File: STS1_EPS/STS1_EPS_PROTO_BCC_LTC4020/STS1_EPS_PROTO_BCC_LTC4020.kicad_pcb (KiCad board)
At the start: 2 copper layers, 47 parts, among them J1 1729267, J10 External Thermistor, J11 Terminal BAT, J9 Output, Q1 SI7135DP-T1-GE3, U1 LTC4020EUHF-PBF, U2 SI7272DP-T1-GE3, U3 SI7272DP-T1-GE3

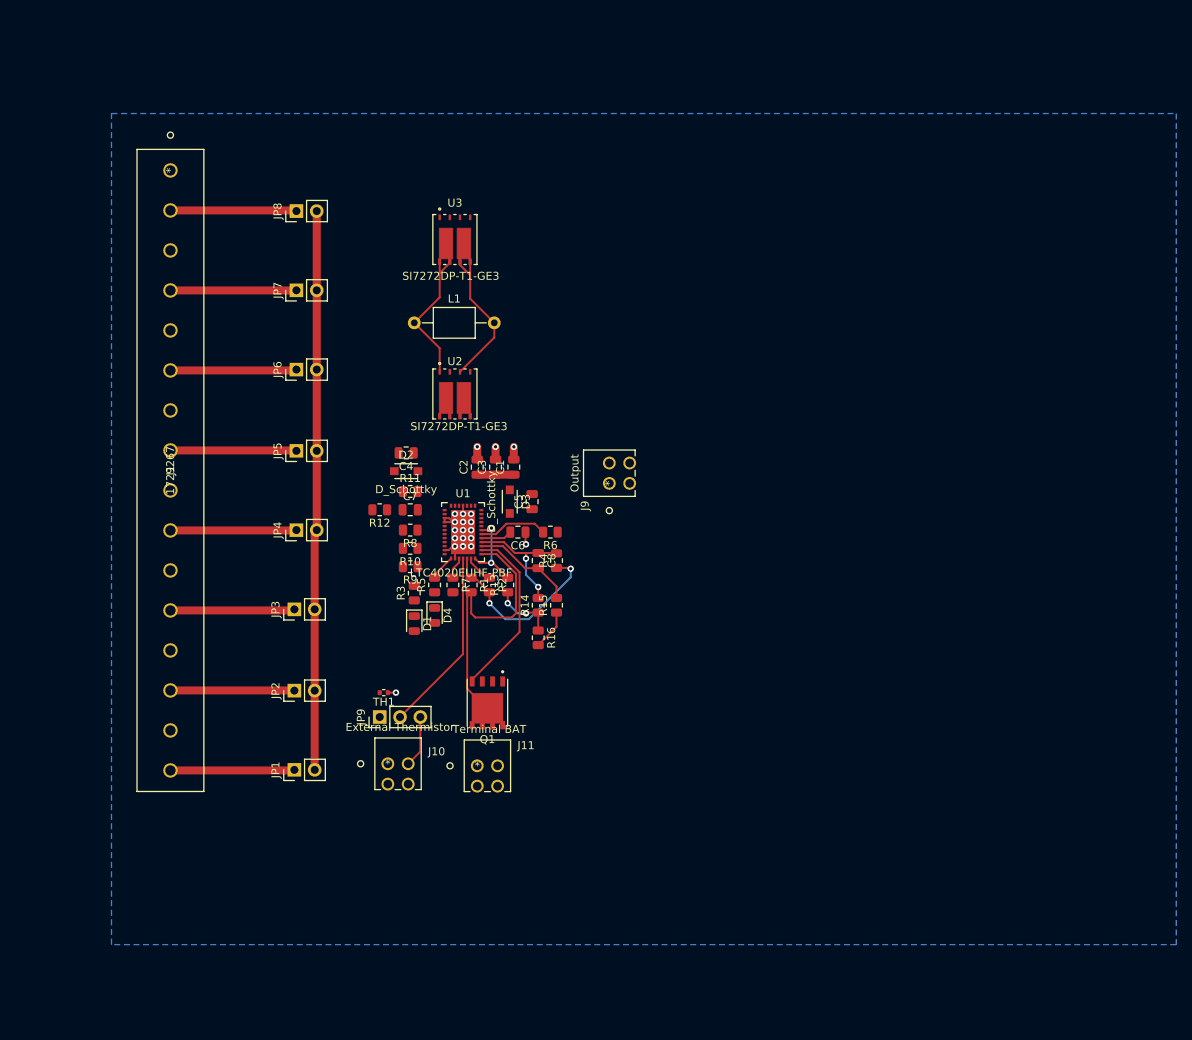
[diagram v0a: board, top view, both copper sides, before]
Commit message: Reworked BCC
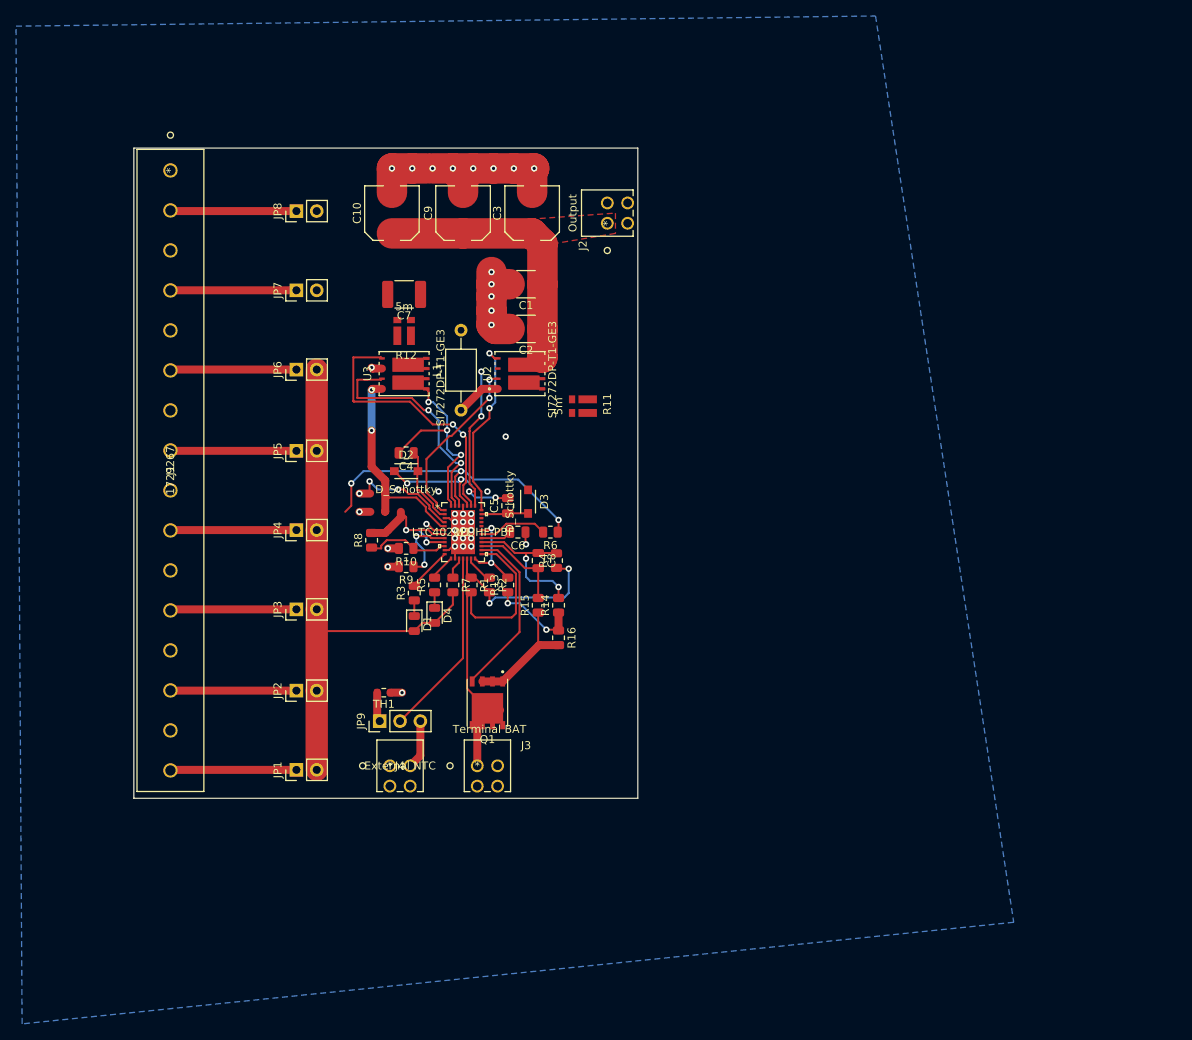
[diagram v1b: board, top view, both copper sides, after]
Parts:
- removed J10: External Thermistor, footprints:1725656
- added C10: 56µ, Capacitor_SMD:C_Elec_6.3x5.4, F.Cu at (89.7, 38.9)
- added C9: 56µ, Capacitor_SMD:C_Elec_6.3x5.4, F.Cu at (98.6, 38.9)
- added J4: External NTC, footprints:1725656, F.Cu at (89.4, 108.0)
- C1, C7: value C -> 100n; footprint Capacitor_SMD:C_0805_2012Metric -> Capacitor_SMD:C_1812_4532Metric
- C2: value C -> 4µ7; footprint Capacitor_SMD:C_0805_2012Metric -> Capacitor_SMD:C_1812_4532Metric
- C3: value CP -> 56µ; footprint Capacitor_SMD:C_0805_2012Metric -> Capacitor_SMD:C_Elec_6.3x5.4
- C4, C5: value C -> 1µ
- L1: value 1m -> INDUCTOR
- R11, R12: value R -> 5m; footprint Resistor_SMD:R_0805_2012Metric -> footprints:CST0612-FC-R002E
- TH1: footprint Resistor_SMD:R_0402_1005Metric -> Resistor_SMD:R_0603_1608Metric
- moved J2 32.5 mm to (116.6, 40.1)
- moved C3 32.1 mm to (107.2, 38.9)
- moved C7 26.9 mm to (91.2, 49.0), turned to 180 degrees
- moved R11 24.1 mm to (113.5, 63.0), turned to 90 degrees
- moved C1 22.9 mm to (106.4, 47.8), turned to 180 degrees
- moved R12 22.6 mm to (91.2, 53.6), turned to 0 degrees
- moved C2 18.3 mm to (106.4, 53.3), turned to 180 degrees
- moved U3 17.9 mm to (91.2, 58.9), turned to 180 degrees
- moved L1 12.4 mm to (98.3, 63.5), turned to 90 degrees
- moved U2 8.52 mm to (105.7, 58.9), turned to 180 degrees
- moved R8 4.99 mm to (87.1, 79.8), turned to 90 degrees
- moved C5 3.09 mm to (104.1, 75.4)
- moved R14 2.54 mm to (110.5, 87.9)
- moved R16 2.54 mm to (110.5, 91.9)
- moved D3 2.29 mm to (106.7, 74.9)
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- renumbered J9 to J2, J11 to J3
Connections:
- C7 pad 2: /EPS Battery Charger/SENSBOT -> Net-(C7-Pad2)
- R11 pad 2: /EPS Battery Charger/SENSTOP -> /EPS Battery Charger/Vin
- R12 pad 1: /EPS Battery Charger/SENSBOT -> Net-(C7-Pad2)
- R12 pad 2: GND -> /EPS Battery Charger/SENSBOT
- U1 pad 28: Net-(U1-Pad28) -> /EPS Battery Charger/Vin
- U1 pad 29: Net-(U1-Pad29) -> GND
- U2 pad 7: /EPS Battery Charger/SENSTOP -> Net-(R11-Pad3)
- U2 pad 8: Net-(U2-Pad8) -> Net-(R11-Pad3)
- U3 pad 1: /EPS Battery Charger/SENSBOT -> Net-(C7-Pad2)
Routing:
- net /EPS Battery Charger/Vin: track 70.0 -> 129.6 mm, vias 0 -> 5
- net GND: track 21.9 -> 74.1 mm, vias 20 -> 37
- net /EPS Battery Charger/BG2: track 0.00 -> 34.1 mm, vias 0 -> 2
- net /EPS Battery Charger/Vout: track 12.6 -> 45.2 mm
- net /EPS Battery Charger/BG1: track 0.00 -> 29.6 mm, vias 0 -> 2
- net /EPS Battery Charger/SENSBOT: track 0.00 -> 26.7 mm, vias 0 -> 2
- net /EPS Battery Charger/TG2: track 0.00 -> 22.8 mm, vias 0 -> 2
- net /EPS Battery Charger/TG1: track 0.00 -> 22.0 mm, vias 0 -> 2
- net /EPS Battery Charger/INTVCC: track 0.00 -> 14.6 mm, vias 0 -> 3
- net /EPS Battery Charger/SW1: track 18.3 -> 31.1 mm, vias 0 -> 3
- net Net-(R10-Pad1): track 0.00 -> 11.3 mm
- net Net-(Q1-Pad1): track 5.01 -> 15.5 mm
- net /EPS Battery Charger/BAT: track 36.7 -> 46.5 mm
- net /EPS Battery Charger/BST1: track 0.00 -> 9.80 mm
- net Net-(R9-Pad1): track 0.00 -> 9.56 mm, vias 0 -> 2
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- added copper zone on F.Cu, net /EPS Battery Charger/Vout
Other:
- board outline added: 63 x 81.3 mm
- net class 6A Power added: clearance 0.2, trace_width 0.25, via_dia 0.8, via_drill 0.4
